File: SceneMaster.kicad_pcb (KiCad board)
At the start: 4 copper layers, 50 x 30 mm, 102 parts, among them J1 TYPE-C-31-M-12, J11 PowerIn, J12 PowerOut, J13 LED3, J14 LED4, J15 LED5, J2 SPK_R, J3 LED1, J4 LED2, J5 LED6, J6 Sensor3, J7 Sensor1, J8 Sensor2, J9 SPK_L, Q1 AO3400A, Q2 AO3400A, Q3 AO3400A, Q4 AO3400A, Q5 AO3400A, Q6 AO3400A, SW1 BUT0, U1 USBLC6-2P6, U2 W25Q128JVS, U3 AMS1117-3.3, U4 STM32F103C8T6, U5 8002B_D, U6 8002B_D, Y1 8MHz

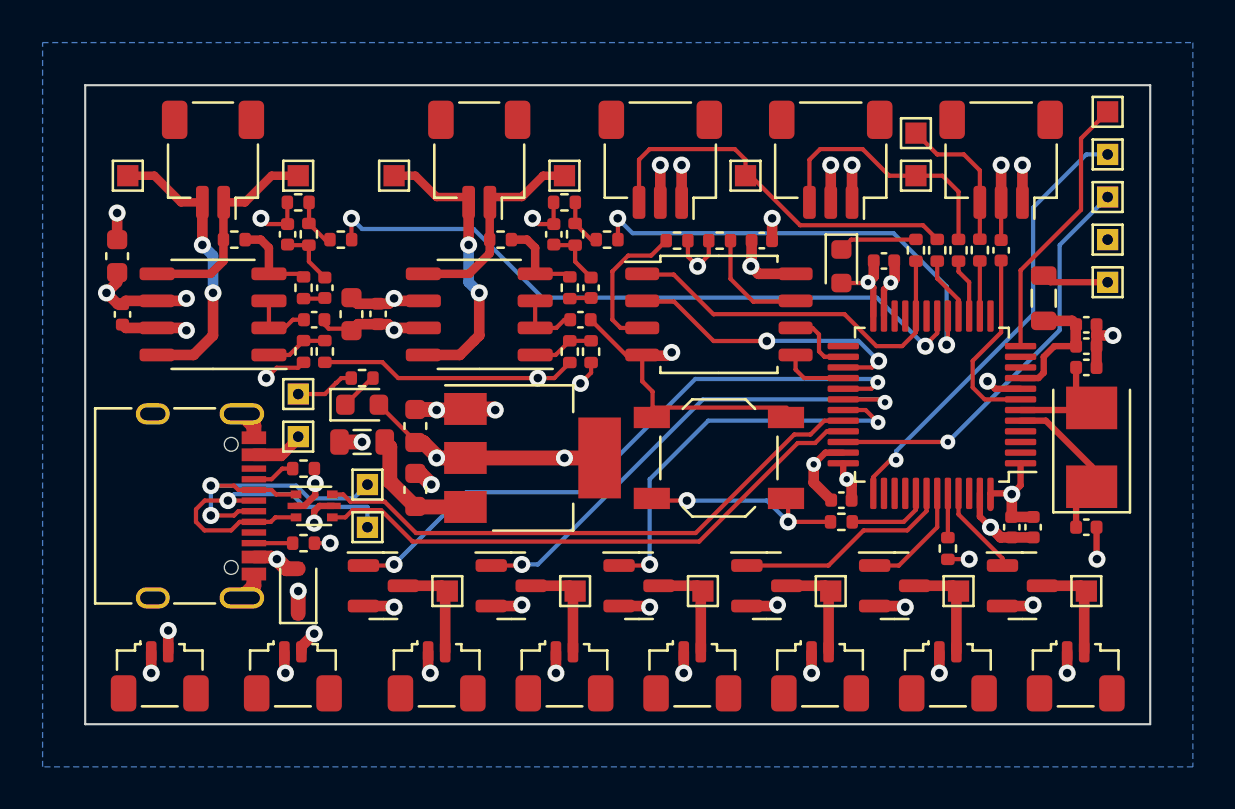
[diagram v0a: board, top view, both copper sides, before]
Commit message: First SGGS re-route
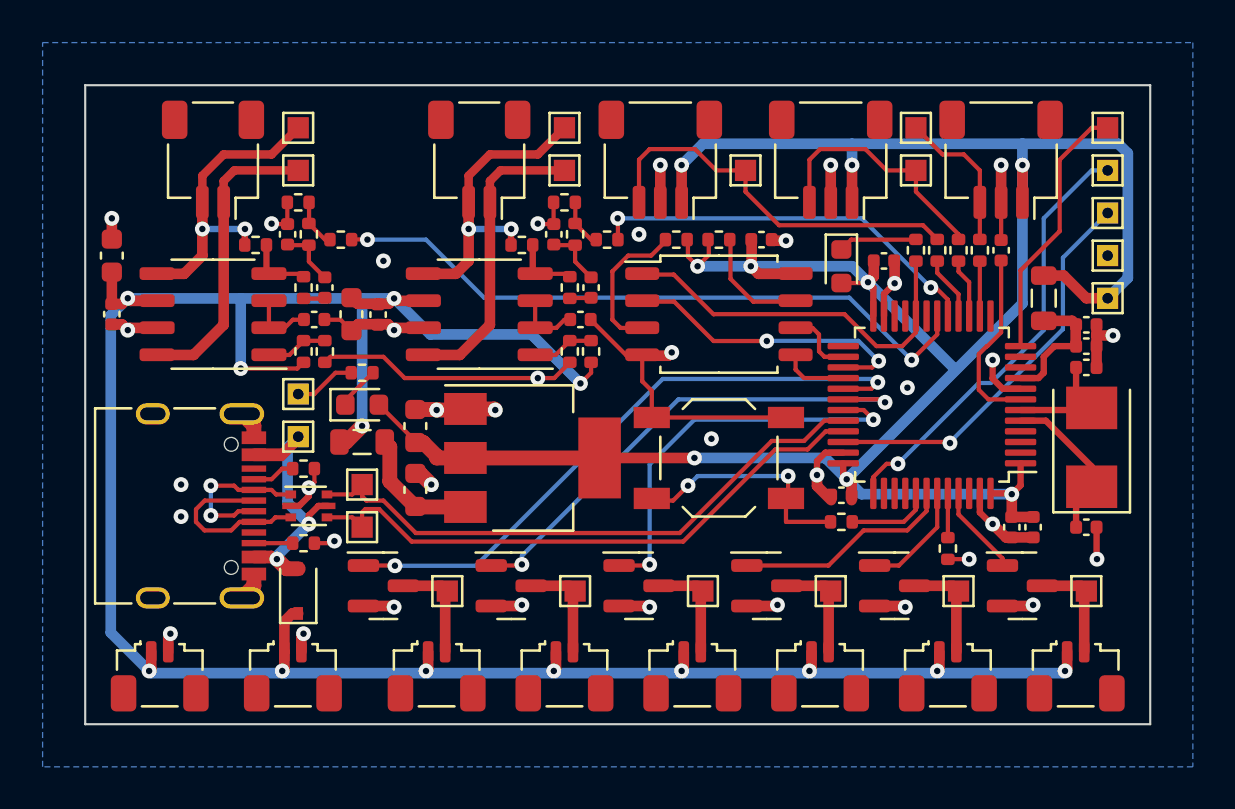
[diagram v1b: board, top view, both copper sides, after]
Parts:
- TP14: value SPK_R+ -> SPK_R-
- TP15: value SKP_L+ -> SKP_L-
- TP21: value SPK_R- -> SPK_R+
- TP22: value SKP_L- -> SKP_L+
- TP6, TP7: footprint TestPoint:TestPoint_THTPad_1.0x1.0mm_Drill0.5mm -> TestPoint:TestPoint_Pad_1.0x1.0mm
- moved TP21 8.31 mm to (122.5, 67.0)
- moved TP22 8.31 mm to (110.0, 67.0)
- moved R21 1.03 mm to (120.5, 72.5)
- moved R25 1.03 mm to (108.0, 72.5)
- moved TP19 0.75 mm to (148.0, 75.0)
- moved TP20 0.75 mm to (148.0, 73.0)
- moved TP3 0.75 mm to (148.0, 69.0)
- moved TP4 0.75 mm to (148.0, 71.0)
- moved TP5 0.75 mm to (148.0, 67.0)
- moved C19 0.50 mm to (101.2, 75.8)
- moved C22 0.25 mm to (101.2, 73.0)
- moved R13 0.25 mm to (113.0, 78.5)
- moved TP1 0.25 mm to (131.0, 69.0)
- moved TP10 0.25 mm to (139.0, 67.0)
- moved TP14 0.25 mm to (122.5, 69.0)
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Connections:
- J2 pad 1: /SPK_R+ -> /SPK_R-
- J2 pad 2: /SPK_R- -> /SPK_R+
- J9 pad 1: /SPK_L+ -> /SPK_L-
- J9 pad 2: /SPK_L- -> /SPK_L+
- TP14 pad 1: /SPK_R+ -> /SPK_R-
- TP15 pad 1: /SPK_L+ -> /SPK_L-
- TP21 pad 1: /SPK_R- -> /SPK_R+
- TP22 pad 1: /SPK_L- -> /SPK_L+
- TP6 pad 1: /D- -> /USB_DN
- TP7 pad 1: /D+ -> /USB_DP
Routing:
- net +5V: track 22.3 -> 117.3 mm, vias 15 -> 13
- net +3V3: track 36.1 -> 118.6 mm, vias 10 -> 9
- net /D+: track 16.5 -> 8.35 mm, vias 1 -> 0
- net /D-: track 15.5 -> 7.42 mm
- net /SPK_L+: track 10.1 -> 14.4 mm, vias 0 -> 2
- net /SPK_R+: track 10.1 -> 14.3 mm, vias 0 -> 2
- net /PWM_AUDIO_R: track 21.9 -> 18.9 mm
- net GND: track 74.6 -> 71.8 mm, vias 30 -> 36
- net Net-(R24-Pad1): track 4.18 -> 2.88 mm
- net Net-(R20-Pad1): track 4.18 -> 2.88 mm
- net /OSC_OUT: track 5.58 -> 4.41 mm
- net Net-(R3-Pad1): track 9.99 -> 11.1 mm
- net /VBUS: track 17.2 -> 16.1 mm
- net /USB_DP: track 26.9 -> 28.0 mm
- net /OSC_IN: track 7.38 -> 6.35 mm
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- added copper zone on In2.Cu, net GND
- removed copper zone on In2.Cu, net +3V3
- removed copper zone on In2.Cu, net +5V
